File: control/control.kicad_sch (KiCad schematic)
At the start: 35 parts, among them J1 AVR-ISP-6, J2 Conn_01x07_Pin, J3 Conn_01x02_Pin, J4 Conn_01x04_Socket, P1 Conn_01x03_Pin, P2 Conn_01x03_Pin, P3 Conn_01x03_Pin, P4 Conn_01x03_Pin, SW1 SW_Push, U2 ATmega328P-A, Y1 16MHz

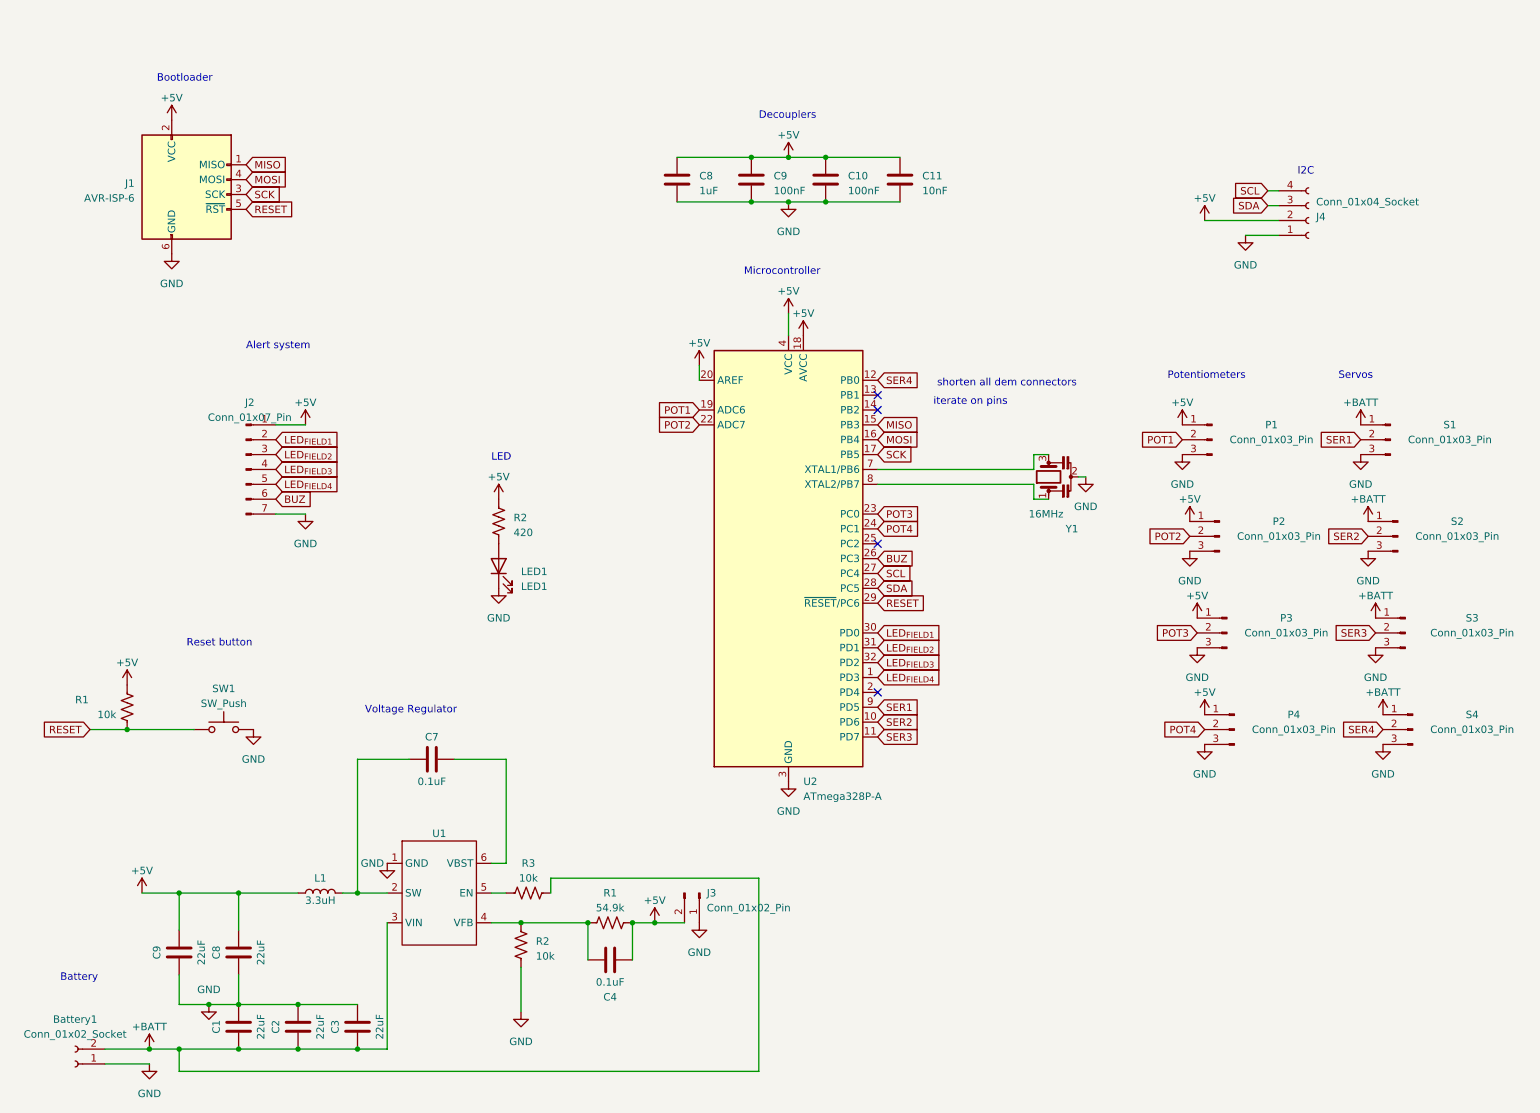
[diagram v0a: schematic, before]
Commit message: Revised hardware
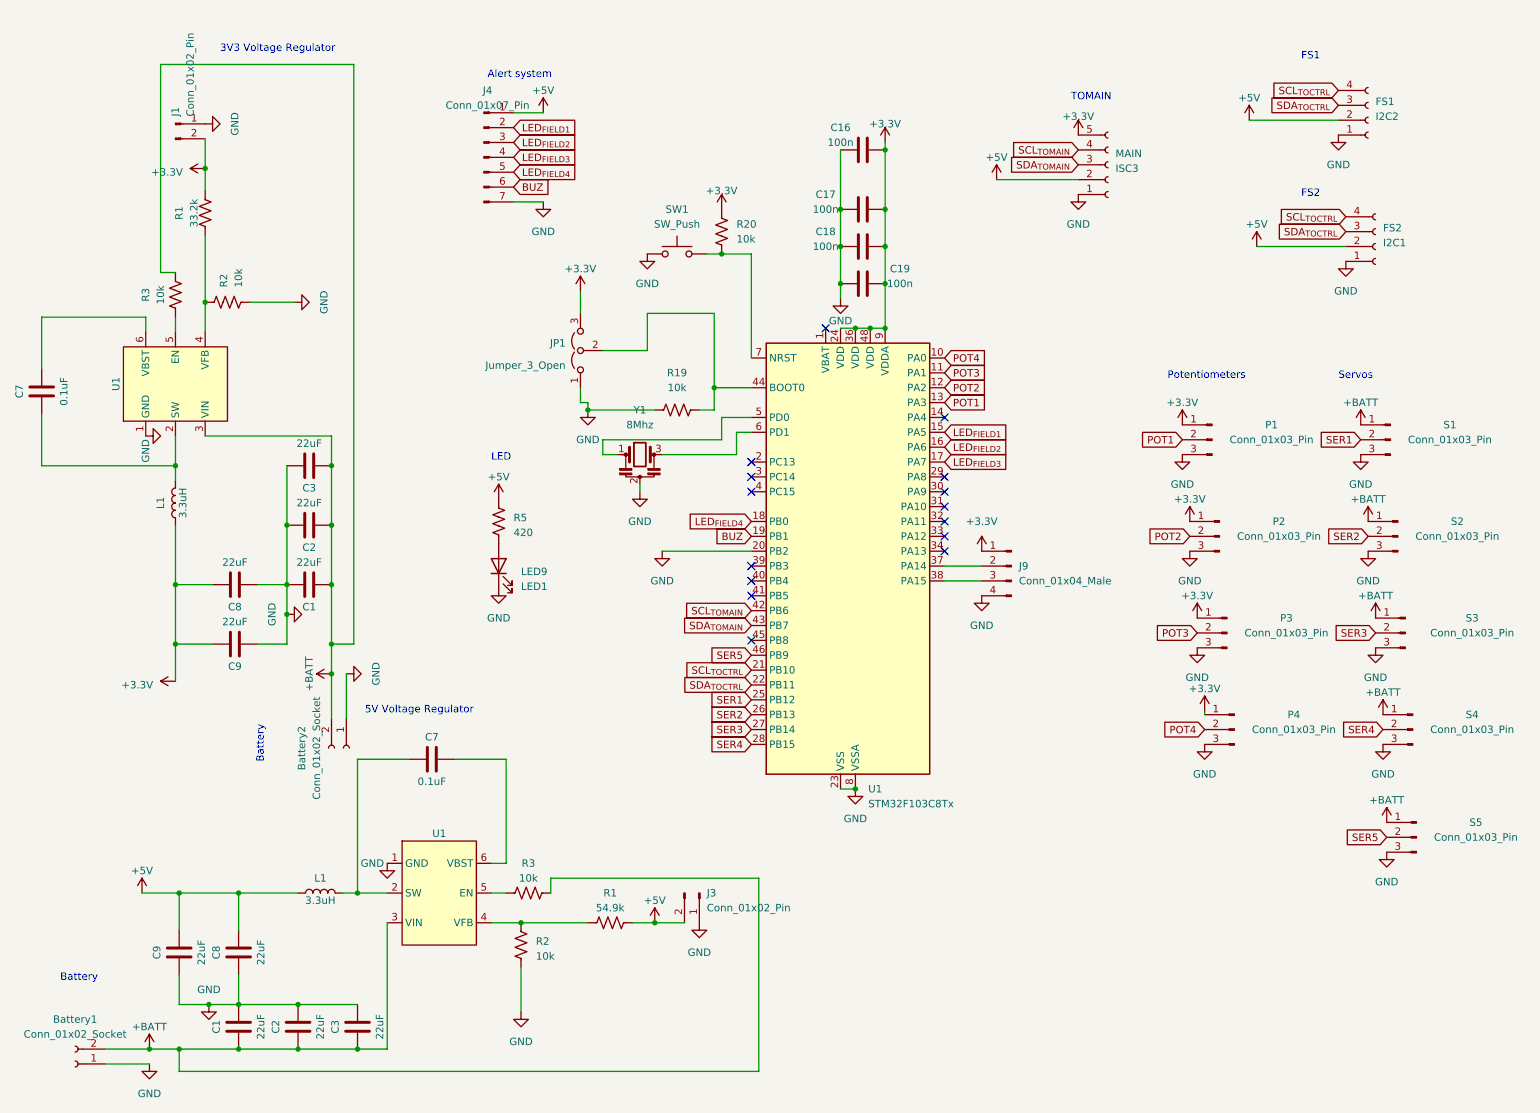
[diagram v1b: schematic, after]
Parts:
- removed C10: 100nF, Capacitor_SMD:C_0805_2012Metric, symbol Device:C
- removed C11: 10nF, Capacitor_SMD:C_0805_2012Metric, symbol Device:C
- removed C4: 0.1uF, Capacitor_SMD:C_0805_2012Metric, symbol Device:C
- removed J1: AVR-ISP-6, Connector_PinHeader_2.54mm:PinHeader_2x03_P2.54mm_Vertical_SMD, symbol Connector:AVR-ISP-6
- removed J4: Conn_01x04_Socket, Connector_JST:JST_XH_B4B-XH-A_1x04_P2.50mm_Vertical, symbol Connector:Conn_01x04_Socket
- removed U2: ATmega328P-A, Package_QFP:TQFP-32_7x7mm_P0.8mm, symbol MCU_Microchip_ATmega:ATmega328P-A
- added Battery2: Conn_01x02_Socket, Connector_Wire:SolderWire-2sqmm_1x02_P7.8mm_D2mm_OD3.9mm, symbol Connector:Conn_01x02_Socket
- added C1, C2, C3: 22uF, Capacitor_SMD:C_0805_2012Metric, symbol Device:C
- added C16, C17, C18, C19: 100n, Capacitor_SMD:C_0603_1608Metric, symbol Device:C
- added C7: 0.1uF, Capacitor_SMD:C_0805_2012Metric, symbol Device:C
- added I2C1: FS2, Connector_JST:JST_XH_B4B-XH-A_1x04_P2.50mm_Vertical, symbol Connector:Conn_01x04_Socket
- added I2C2: FS1, Connector_JST:JST_XH_B4B-XH-A_1x04_P2.50mm_Vertical, symbol Connector:Conn_01x04_Socket
- added ISC3: MAIN, Connector_JST:JST_XH_B5B-XH-A_1x05_P2.50mm_Vertical, symbol Connector:Conn_01x05_Socket
- added J1: Conn_01x02_Pin, Connector_JST:JST_XH_B2B-XH-A_1x02_P2.50mm_Vertical, symbol Connector:Conn_01x02_Pin
- added J9: Conn_01x04_Male, Connector_PinHeader_2.54mm:PinHeader_1x04_P2.54mm_Horizontal, symbol Connector:Conn_01x04_Male
- added JP1: Jumper_3_Open, Jumper:SolderJumper-3_P2.0mm_Open_TrianglePad1.0x1.5mm, symbol Jumper:Jumper_3_Open
- added L1: 3.3uH, Inductor_SMD:L_Taiyo-Yuden_NR-60xx, symbol Device:L
- added R19, R2, R20, R3: 10k, Resistor_SMD:R_0603_1608Metric, symbol Device:R_US
- added S5: Conn_01x03_Pin, Connector_JST:JST_EH_B3B-EH-A_1x03_P2.50mm_Vertical, symbol Connector:Conn_01x03_Pin
- added U1: ~, Package_TO_SOT_SMD:TSOT-23-6, symbol Regulators:TPS563208DDCR
- added U1: STM32F103C8Tx, Package_QFP:LQFP-48_7x7mm_P0.5mm, symbol MCU_ST_STM32F1:STM32F103C8Tx
- C8: value 1uF -> 22uF
- C9: value 100nF -> 22uF
- R1: value 10k -> 33.2k
- SW1: footprint Button_Switch_SMD:SW_SPST_SKQG_WithoutStem -> Button_Switch_SMD:SW_SPST_B3U-1000P-B
- Y1: value 16MHz -> 8Mhz
- renumbered J2 to J4, LED1 to LED9, R2 to R5
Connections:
- net +5V: now also I2C1.2 (Pin_2), I2C2.2 (Pin_2), ISC3.2 (Pin_2); no longer C8.1, C9.1, P1.1 (Pin_1), P2.1 (Pin_1), P3.1 (Pin_1), P4.1 (Pin_1), R1.2
- net +BATT: now also Battery2.2 (Pin_2), C1.1, C2.1, C3.1, R3.2, S5.1 (Pin_1), U1.3 (VIN)
- net BUZ: now also U1.19 (PB1)
- net GND: now also C8.1, C9.1, SW1.1, Battery2.1 (Pin_1), C1.2, C16.1, C17.1, C18.1, C19.2, C2.2, C3.2, I2C1.1 (Pin_1), I2C2.1 (Pin_1), ISC3.1 (Pin_1), J1.1 (Pin_1), J9.4 (Pin_4), JP1.1 (A), R19.1, R2.1, S5.3 (Pin_3), U1.1 (GND), U1.20 (PB2), U1.23 (VSS), U1.35 (VSS), U1.47 (VSS), U1.8 (VSSA); no longer C8.2, C9.2, SW1.2
- net LED_{FIELD1}: now also U1.15 (PA5)
- net LED_{FIELD2}: now also U1.16 (PA6)
- net LED_{FIELD3}: now also U1.17 (PA7)
- net LED_{FIELD4}: now also U1.18 (PB0)
- net POT1: now also U1.13 (PA3)
- net POT2: now also U1.12 (PA2)
- net POT3: now also U1.11 (PA1)
- net POT4: now also U1.10 (PA0)
- net SER1: now also U1.25 (PB12)
- net SER2: now also U1.26 (PB13)
- net SER3: now also U1.27 (PB14)
- net SER4: now also U1.28 (PB15)
- net at Y1.1: now also U1.5 (PD0)
- net at Y1.3: now also U1.6 (PD1)
- net RESET renamed +3.3V
- net +3.3V: now also C8.2, C9.2, P1.1 (Pin_1), P2.1 (Pin_1), P3.1 (Pin_1), P4.1 (Pin_1), C16.2, C17.2, C18.2, C19.1, ISC3.5 (Pin_5), J1.2 (Pin_2), J9.1 (Pin_1), JP1.3 (B), L1.1, R20.1, U1.24 (VDD), U1.36 (VDD), U1.48 (VDD), U1.9 (VDDA); no longer SW1.1
- new net: C7.1, L1.2, U1.2 (SW)
- new net: C7.2, U1.6 (VBST)
- new net: R20.2, SW1.2, U1.7 (NRST)
- new net: JP1.2 (C), R19.2, U1.44 (BOOT0)
- new net: R3.1, U1.5 (EN)
- new net: R1.2, R2.2, U1.4 (VFB)
- new net: J9.2 (Pin_2), U1.37 (PA14)
- new net: J9.3 (Pin_3), U1.38 (PA15)
- new net SCL_{TOCTRL}: I2C1.4 (Pin_4), I2C2.4 (Pin_4), U1.21 (PB10)
- new net SCL_{TOMAIN}: ISC3.4 (Pin_4), U1.42 (PB6)
- new net SDA_{TOCTRL}: I2C1.3 (Pin_3), I2C2.3 (Pin_3), U1.22 (PB11)
- new net SDA_{TOMAIN}: ISC3.3 (Pin_3), U1.43 (PB7)
- new net SER5: S5.2 (Pin_2), U1.46 (PB9)
- no-connect marks 4 -> 15
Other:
- note added: "3V3 Voltage Regulator"
- note added: "5V Voltage Regulator"
- note added: "FS1"
- note added: "FS2"
- note added: "TOMAIN"
- note removed: "Bootloader"
- note removed: "Decouplers"
- note removed: "I2C"
- note removed: "Microcontroller"
- note removed: "Reset button"
- note removed: "Voltage Regulator"
- note removed: "iterate on pins"
- note removed: "shorten all dem connectors"
- moved on the sheet: J4
